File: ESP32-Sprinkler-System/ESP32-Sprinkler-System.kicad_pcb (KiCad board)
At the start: 2 copper layers, 207 x 158.8 mm, 58 parts, among them J101 12V, J102 DHT, J103 NEOPIXEL, J104 LCD, J105 BME280, J201 TBL004-508-02BE-2GY, J202 TBL004-508-02BE-2GY, J203 TBL004-508-02BE-2GY, J204 TBL004-508-02BE-2GY, Q201 IRFZ24NPBF, Q202 IRFZ24NPBF, Q203 IRFZ24NPBF, Q204 IRFZ24NPBF, U101 V7805-500, U102 ESP32-DEVKITC-32D, U201 MC33152PG, U202 MC33152PG

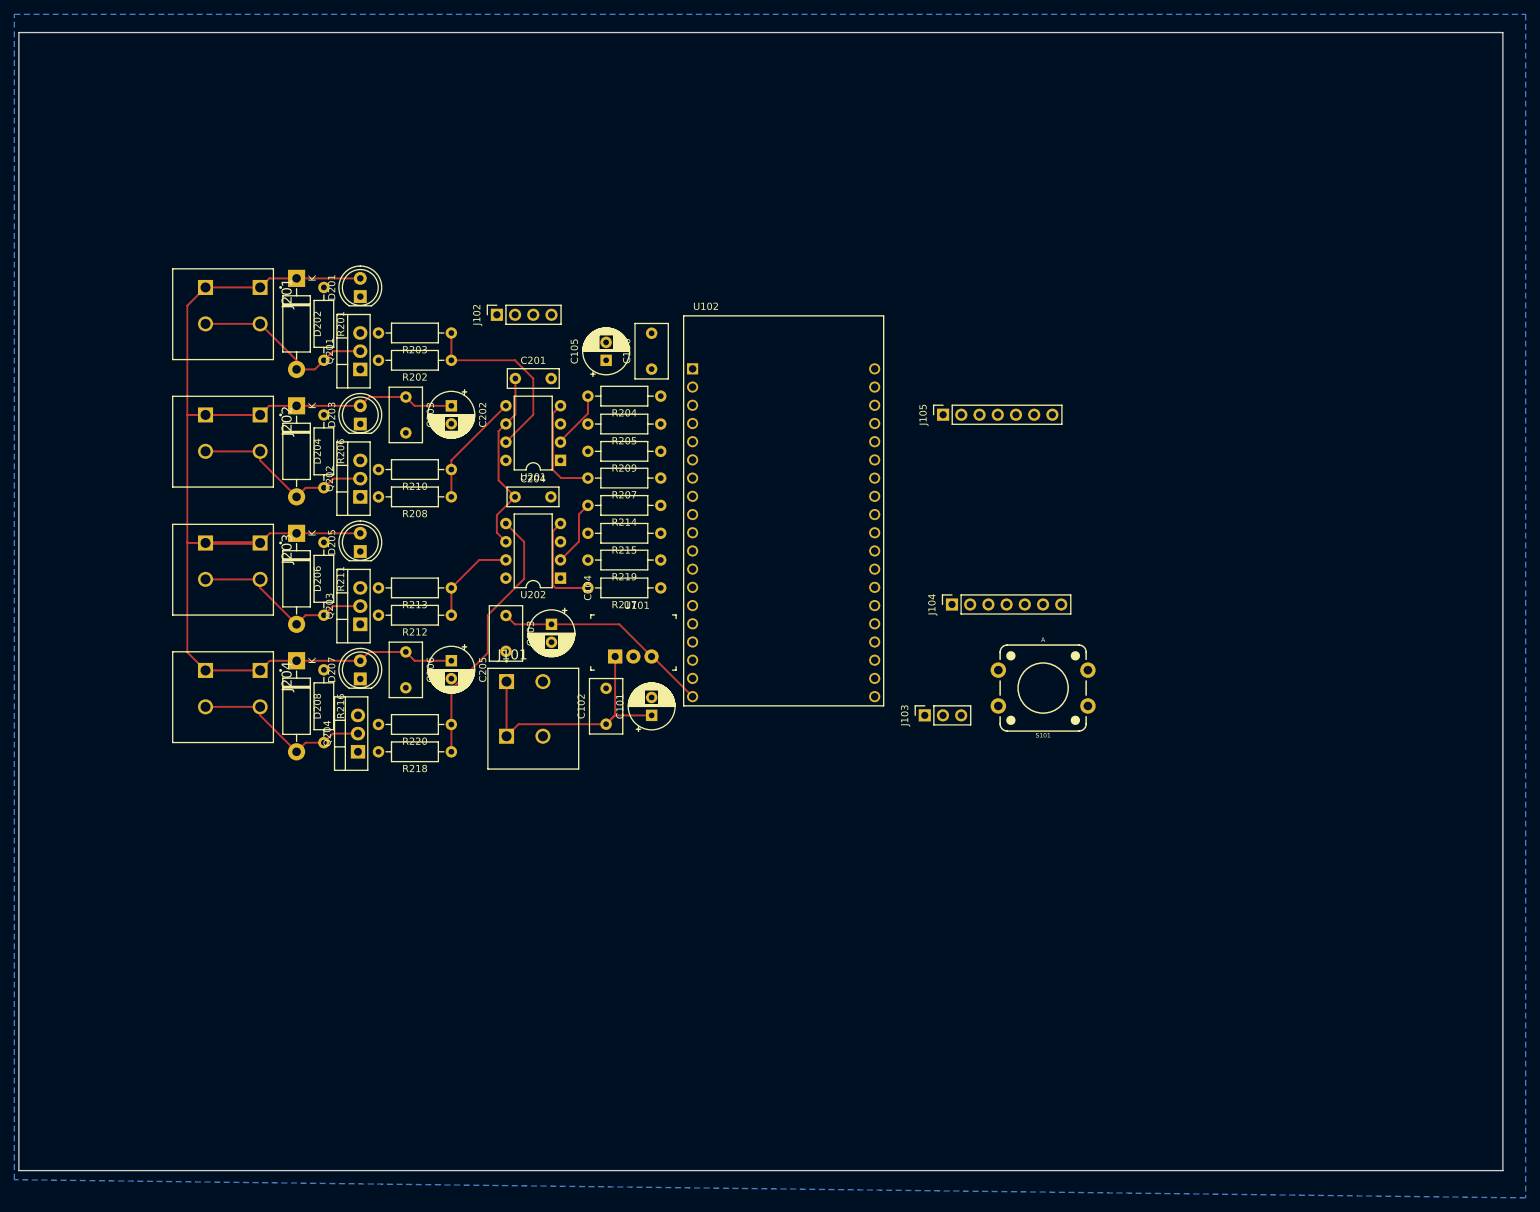
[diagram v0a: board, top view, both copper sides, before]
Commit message: Traces complete
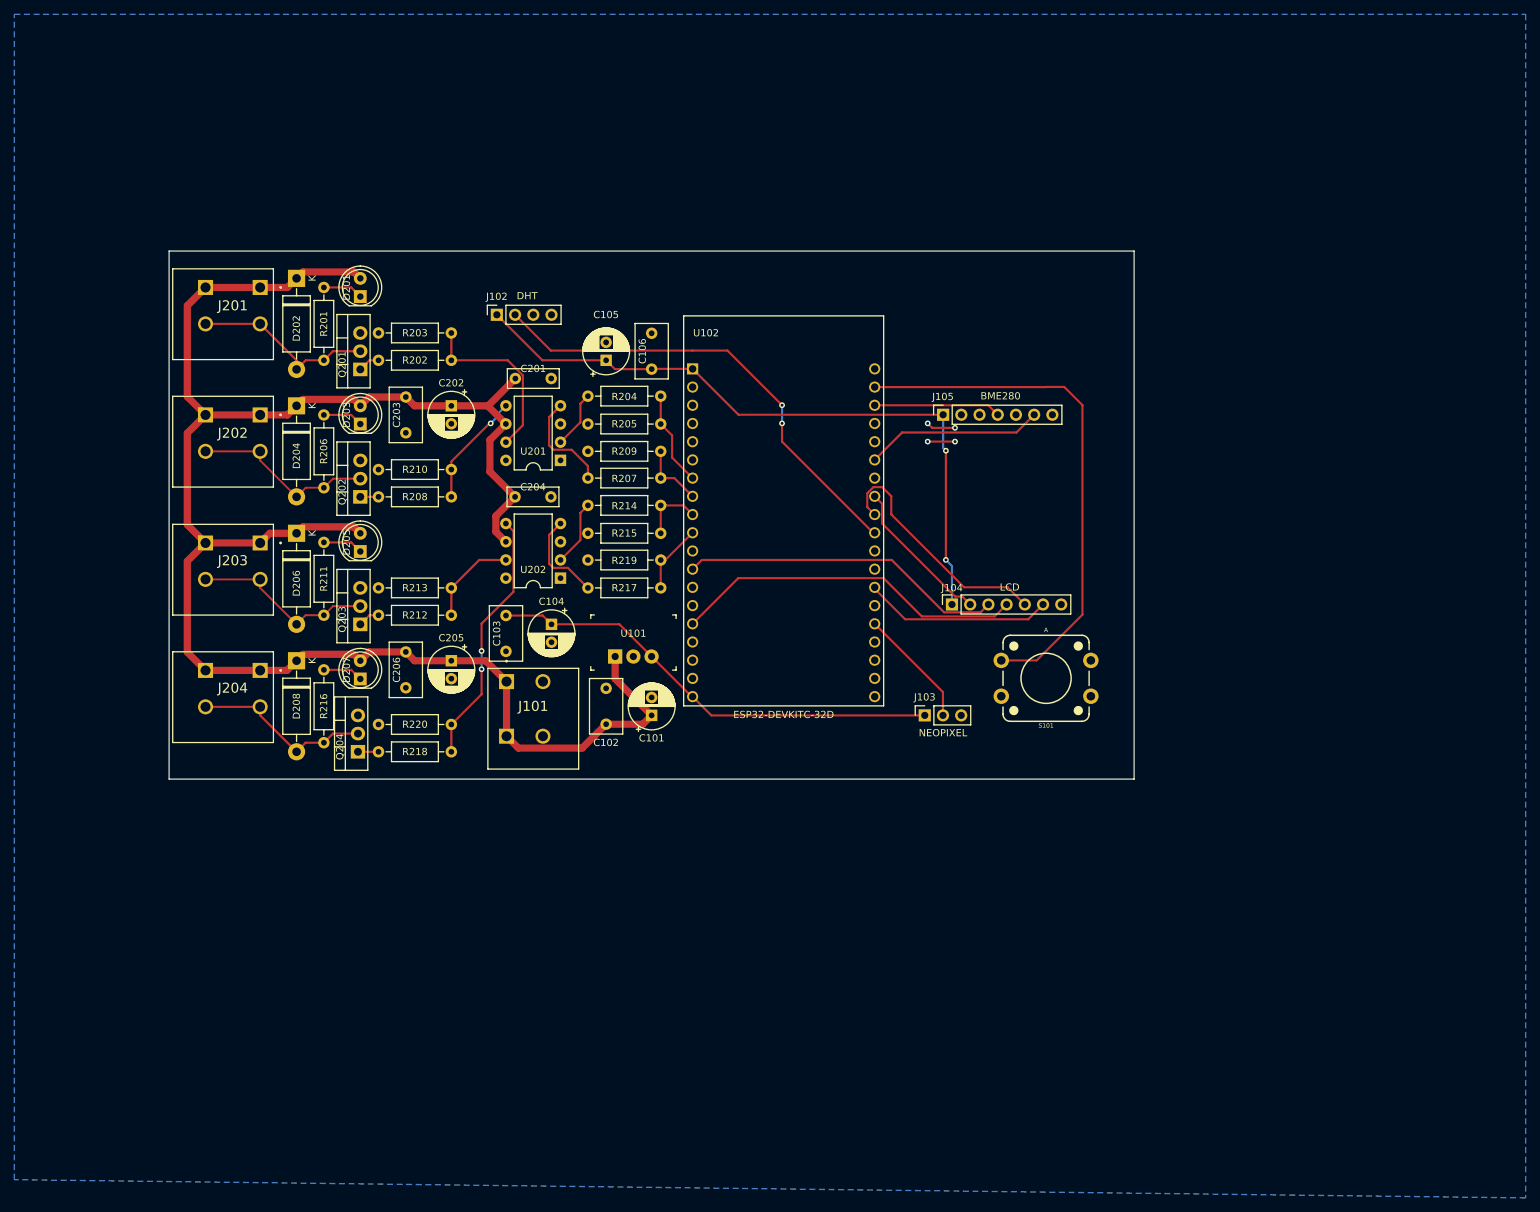
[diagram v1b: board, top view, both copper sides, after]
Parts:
- moved S101 1.42 mm to (180.3, 120.7)
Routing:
- net 3.3V: track 0.00 -> 95.0 mm, vias 0 -> 2
- net SW_A: track 0.00 -> 73.2 mm
- net DHT: track 0.00 -> 65.7 mm, vias 0 -> 2
- net MOSI: track 0.00 -> 49.3 mm
- net SCK: track 0.00 -> 45.3 mm
- net D/C: track 0.00 -> 34.0 mm
- net 5V: track 30.7 -> 64.2 mm
- net BACKLIGHT: track 0.00 -> 26.3 mm
- net SDA: track 0.00 -> 24.9 mm
- net CS: track 0.00 -> 21.2 mm
- net 12V: track 241.9 -> 262.9 mm
- net SCL: track 0.00 -> 17.7 mm
- net NEOPIXEL: track 0.00 -> 16.7 mm
- net Valve1: track 0.00 -> 13.3 mm
- net Valve4: track 0.00 -> 9.91 mm
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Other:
- board size 207 x 158.8 mm -> 134.6 x 73.7 mm

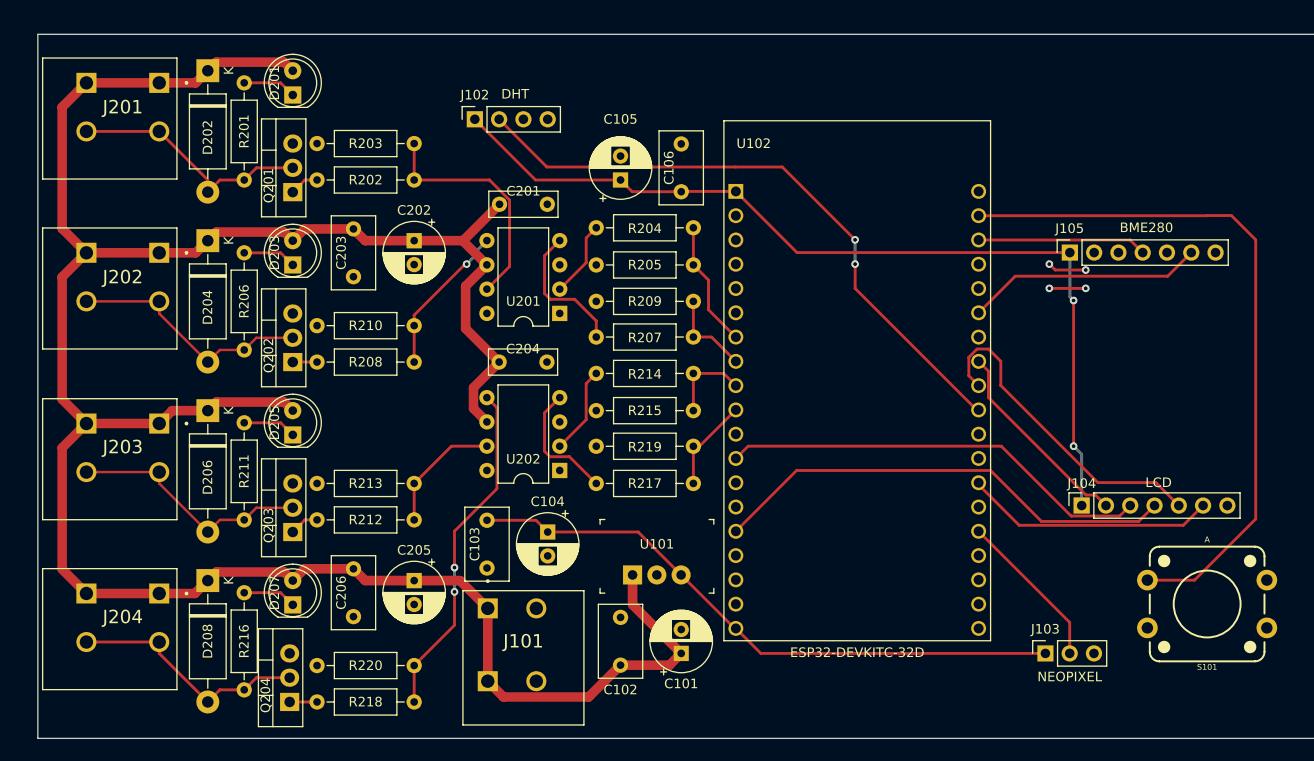
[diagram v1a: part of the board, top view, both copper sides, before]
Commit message: curvy 2 saved
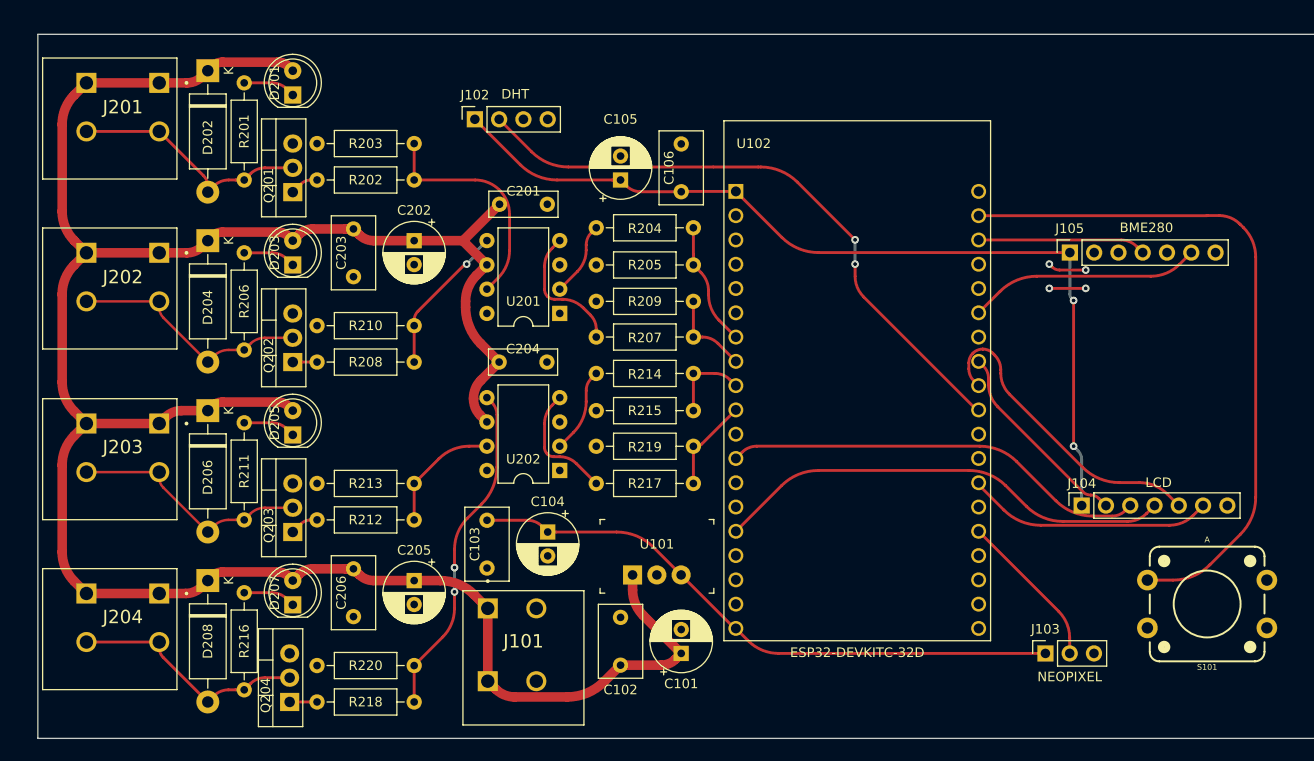
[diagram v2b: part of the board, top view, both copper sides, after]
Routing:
- net 12V: track 262.9 -> 257.8 mm
- net D/C: track 34.0 -> 33.0 mm
- net MOSI: track 49.3 -> 48.4 mm
- net SW_A: track 73.2 -> 72.3 mm
- net 3.3V: track 95.0 -> 94.2 mm
- net Net-(R218-Pad1): track 35.9 -> 35.1 mm
- net SCK: track 45.3 -> 44.6 mm
- net 5V: track 64.2 -> 63.5 mm
- net DHT: track 65.7 -> 65.1 mm
- net Net-(D206-Pad2): track 25.9 -> 25.3 mm
- net Net-(R202-Pad1): track 25.0 -> 24.4 mm
